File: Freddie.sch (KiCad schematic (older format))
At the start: 14 parts, among them J100 cond, J101 cond, U18 74LS08, U6 Freddie, Y1 Crystal

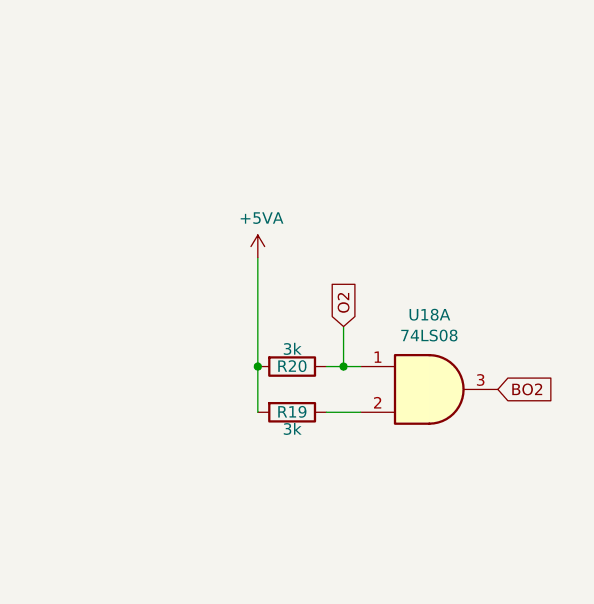
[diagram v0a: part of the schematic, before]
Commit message: GTIA
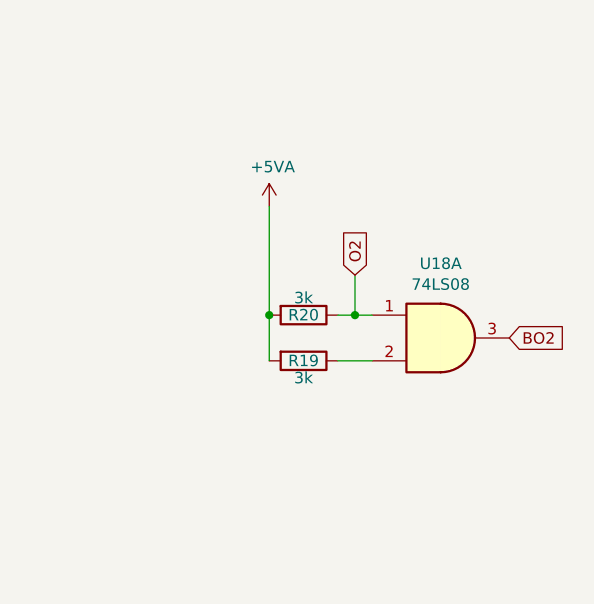
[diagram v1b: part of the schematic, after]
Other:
- moved on the sheet: R19, R20, U18A
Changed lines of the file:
@@
 $Descr A4 11693 8268
 encoding utf-8
-Sheet 5 13
+Sheet 5 14
 Title ""
 Date ""
@@
 L 74xx:74LS08 U18
 U 1 1 60220D8B
-P 8900 3025
-F 0 "U18" H 8900 3350 50  0000 C CNN
-F 1 "74LS08" H 8900 3259 50  0000 C CNN
-F 2 "Package_DIP:DIP-14_W7.62mm_Socket" H 8900 3025 50  0001 C CNN
-F 3 "http://www.ti.com/lit/gpn/sn74LS08" H 8900 3025 50  0001 C CNN
-	1    8900 3025
+P 8950 2800
+F 0 "U18" H 8950 3125 50  0000 C CNN
+F 1 "74LS08" H 8950 3034 50  0000 C CNN
+F 2 "Package_DIP:DIP-14_W7.62mm_Socket" H 8950 2800 50  0001 C CNN
+F 3 "http://www.ti.com/lit/gpn/sn74LS08" H 8950 2800 50  0001 C CNN
+	1    8950 2800
 	1    0    0    -1
 $EndComp
@@
 L Device:R R19
 U 1 1 602255FA
-P 8300 3125
-F 0 "R19" V 8300 3125 50  0000 C CNN
-F 1 "3k" V 8375 3125 50  0000 C CNN
-F 2 "Atari:R_Axial_DIN0207_L3.6mm_D2.2mm_P10.16mm_Horizontal" V 8230 3125 50  0001 C CNN
-F 3 "~" H 8300 3125 50  0001 C CNN
-	1    8300 3125
+P 8350 2900
+F 0 "R19" V 8350 2900 50  0000 C CNN
+F 1 "3k" V 8425 2900 50  0000 C CNN
+F 2 "Atari:R_Axial_DIN0207_L3.6mm_D2.2mm_P10.16mm_Horizontal" V 8280 2900 50  0001 C CNN
+F 3 "~" H 8350 2900 50  0001 C CNN
+	1    8350 2900
 	0    1    1    0
 $EndComp
@@
 L Device:R R20
 U 1 1 60225F1A
-P 8300 2925
-F 0 "R20" V 8300 2925 50  0000 C CNN
-F 1 "3k" V 8225 2925 50  0000 C CNN
-F 2 "Atari:R_Axial_DIN0207_L3.6mm_D2.2mm_P10.16mm_Horizontal" V 8230 2925 50  0001 C CNN
-F 3 "~" H 8300 2925 50  0001 C CNN
-	1    8300 2925
-	0    1    1    0
-$EndComp
-Wire Wire Line
-	8450 2925 8525 2925
-Text GLabel 9200 3025 2    50   Input ~ 0
+P 8350 2700
+F 0 "R20" V 8350 2700 50  0000 C CNN
+F 1 "3k" V 8275 2700 50  0000 C CNN
+F 2 "Atari:R_Axial_DIN0207_L3.6mm_D2.2mm_P10.16mm_Horizontal" V 8280 2700 50  0001 C CNN
+F 3 "~" H 8350 2700 50  0001 C CNN
+	1    8350 2700
+	0    1    1    0
+$EndComp
+Wire Wire Line
+	8500 2700 8575 2700
+Text GLabel 9250 2800 2    50   Input ~ 0
 BO2
 Wire Wire Line
-	8150 3125 8150 2925
+	8200 2900 8200 2700
 $Comp
 L power:+5VA #PWR0142
 U 1 1 602274F9
-P 8150 2450
-F 0 "#PWR0142" H 8150 2300 50  0001 C CNN
-F 1 "+5VA" H 8165 2623 50  0000 C CNN
-F 2 "" H 8150 2450 50  0001 C CNN
-F 3 "" H 8150 2450 50  0001 C CNN
-	1    8150 2450
-	1    0    0    -1
-$EndComp
-Wire Wire Line
-	8150 2450 8150 2925
-Connection ~ 8150 2925
-Text GLabel 8525 2750 1    50   Input ~ 0
+P 8200 2225
+F 0 "#PWR0142" H 8200 2075 50  0001 C CNN
+F 1 "+5VA" H 8215 2398 50  0000 C CNN
+F 2 "" H 8200 2225 50  0001 C CNN
+F 3 "" H 8200 2225 50  0001 C CNN
+	1    8200 2225
+	1    0    0    -1
+$EndComp
+Wire Wire Line
+	8200 2225 8200 2700
+Connection ~ 8200 2700
+Text GLabel 8575 2525 1    50   Input ~ 0
 O2
 Wire Wire Line
-	8450 3125 8600 3125
-Wire Wire Line
-	8525 2750 8525 2925
-Connection ~ 8525 2925
-Wire Wire Line
-	8525 2925 8600 2925
+	8500 2900 8650 2900
+Wire Wire Line
+	8575 2525 8575 2700
+Connection ~ 8575 2700
+Wire Wire Line
+	8575 2700 8650 2700
 $Comp
 L Connector_Generic:Conn_01x01 J100

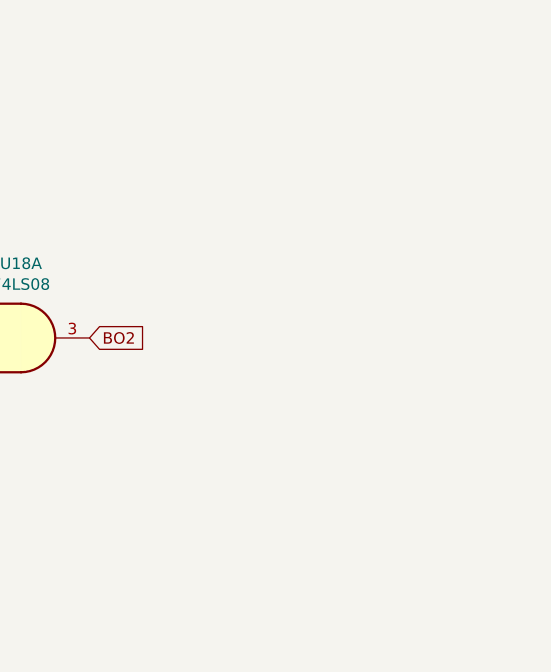
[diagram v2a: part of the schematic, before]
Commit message: Schema finished
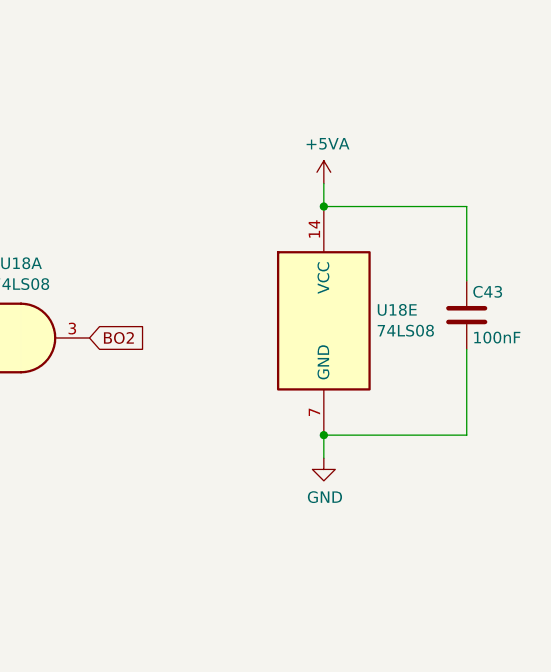
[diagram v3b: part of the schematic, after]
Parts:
- added C43: 100nF, Atari:C_Axial_L5.1mm_D2.5mm_P12.50mm_Horizontal, symbol Device:C
- added unit 5 of U18
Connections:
- net +5VA: now also C43.1, U18.14 (VCC)
- net GND: now also C43.2, U18.7 (GND)
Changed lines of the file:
@@
 	4200 1825 4200 2575
 Connection ~ 2950 1825
+$Comp
+L 74xx:74LS08 U18
+U 5 1 603127C5
+P 10275 2725
+F 0 "U18" H 10505 2771 50  0000 L CNN
+F 1 "74LS08" H 10505 2680 50  0000 L CNN
+F 2 "Package_DIP:DIP-14_W7.62mm_Socket" H 10275 2725 50  0001 C CNN
+F 3 "http://www.ti.com/lit/gpn/sn74LS08" H 10275 2725 50  0001 C CNN
+	5    10275 2725
+	1    0    0    -1
+$EndComp
+$Comp
+L power:+5VA #PWR0235
+U 1 1 60314A8A
+P 10275 2125
+F 0 "#PWR0235" H 10275 1975 50  0001 C CNN
+F 1 "+5VA" H 10290 2298 50  0000 C CNN
+F 2 "" H 10275 2125 50  0001 C CNN
+F 3 "" H 10275 2125 50  0001 C CNN
+	1    10275 2125
+	1    0    0    -1
+$EndComp
+Wire Wire Line
+	10275 2125 10275 2225
+$Comp
+L power:GND #PWR0236
+U 1 1 6031559C
+P 10275 3325
+F 0 "#PWR0236" H 10275 3075 50  0001 C CNN
+F 1 "GND" H 10280 3152 50  0000 C CNN
+F 2 "" H 10275 3325 50  0001 C CNN
+F 3 "" H 10275 3325 50  0001 C CNN
+	1    10275 3325
+	1    0    0    -1
+$EndComp
+Wire Wire Line
+	10275 3225 10275 3325
+$Comp
+L Device:C C43
+U 1 1 603176DF
+P 10900 2700
+F 0 "C43" H 10925 2800 50  0000 L CNN
+F 1 "100nF" H 10925 2600 50  0000 L CNN
+F 2 "Atari:C_Axial_L5.1mm_D2.5mm_P12.50mm_Horizontal" H 10938 2550 50  0001 C CNN
+F 3 "~" H 10900 2700 50  0001 C CNN
+	1    10900 2700
+	1    0    0    -1
+$EndComp
+Wire Wire Line
+	10275 2225 10900 2225
+Wire Wire Line
+	10900 2225 10900 2550
+Connection ~ 10275 2225
+Wire Wire Line
+	10275 3225 10900 3225
+Wire Wire Line
+	10900 3225 10900 2850
+Connection ~ 10275 3225
 $EndSCHEMATC

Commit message: Tracking
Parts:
- R18, R26: footprint Atari:R_Axial_DIN0207_L3.6mm_D2.2mm_P10.16mm_Horizontal -> Resistor_THT:R_Axial_DIN0207_L6.3mm_D2.5mm_P10.16mm_Horizontal
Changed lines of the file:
@@
 F 0 "R18" V 3843 1825 50  0000 C CNN
 F 1 "240" V 3934 1825 50  0000 C CNN
-F 2 "Atari:R_Axial_DIN0207_L3.6mm_D2.2mm_P10.16mm_Horizontal" V 3980 1825 50  0001 C CNN
+F 2 "Resistor_THT:R_Axial_DIN0207_L6.3mm_D2.5mm_P10.16mm_Horizontal" V 3980 1825 50  0001 C CNN
 F 3 "~" H 4050 1825 50  0001 C CNN
 	1    4050 1825
@@
 F 0 "R26" V 3843 2575 50  0000 C CNN
 F 1 "1M" V 3934 2575 50  0000 C CNN
-F 2 "Atari:R_Axial_DIN0207_L3.6mm_D2.2mm_P10.16mm_Horizontal" V 3980 2575 50  0001 C CNN
+F 2 "Resistor_THT:R_Axial_DIN0207_L6.3mm_D2.5mm_P10.16mm_Horizontal" V 3980 2575 50  0001 C CNN
 F 3 "~" H 4050 2575 50  0001 C CNN
 	1    4050 2575

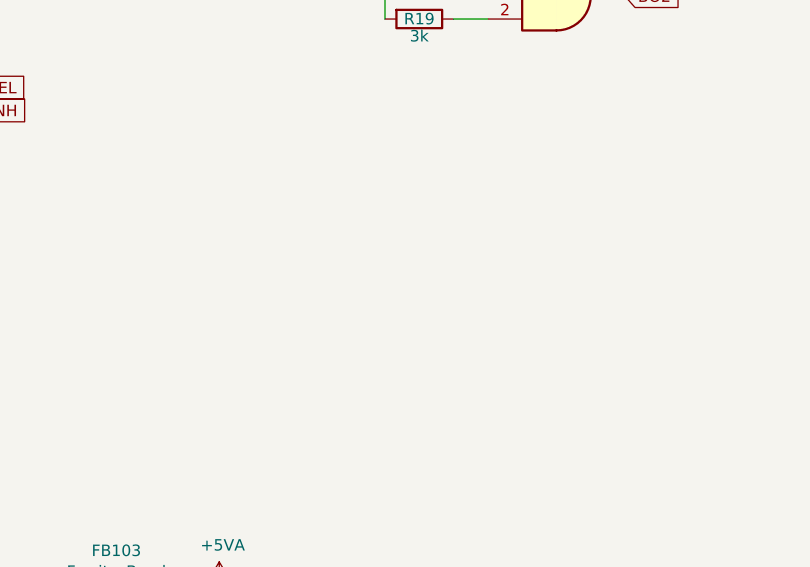
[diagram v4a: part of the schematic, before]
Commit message: Trackimg
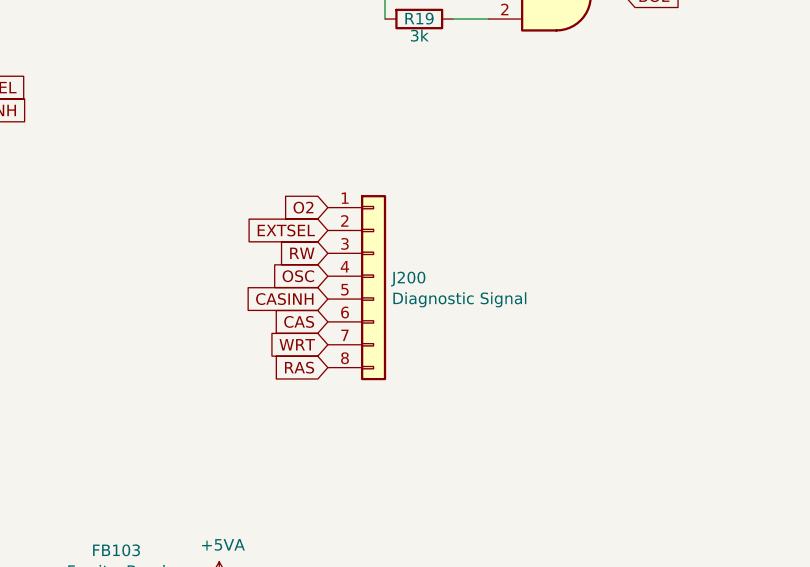
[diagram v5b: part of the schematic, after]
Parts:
- added J200: Diagnostic Signal, Connector_PinHeader_2.54mm:PinHeader_1x08_P2.54mm_Vertical, symbol Connector_Generic:Conn_01x08
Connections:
- net CAS: now also J200.6 (Pin_6)
- net CASINH: now also J200.5 (Pin_5)
- net EXTSEL: now also J200.2 (Pin_2)
- net O2: now also J200.1 (Pin_1)
- net OSC: now also J200.4 (Pin_4)
- net RAS: now also J200.8 (Pin_8)
- net RW: now also J200.3 (Pin_3)
- net WRT: now also J200.7 (Pin_7)
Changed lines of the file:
@@
 	10900 3225 10900 2850
 Connection ~ 10275 3225
+$Comp
+L Connector_Generic:Conn_01x08 J200
+U 1 1 60415DC7
+P 8150 4025
+F 0 "J200" H 8230 4017 50  0000 L CNN
+F 1 "Diagnostic Signal" H 8230 3926 50  0000 L CNN
+F 2 "Connector_PinHeader_2.54mm:PinHeader_1x08_P2.54mm_Vertical" H 8150 4025 50  0001 C CNN
+F 3 "~" H 8150 4025 50  0001 C CNN
+	1    8150 4025
+	1    0    0    -1
+$EndComp
+Text GLabel 7950 4225 0    50   Input ~ 0
+CAS
+Text GLabel 7950 4325 0    50   Input ~ 0
+WRT
+Text GLabel 7950 4425 0    50   Input ~ 0
+RAS
+Text GLabel 7950 3925 0    50   Input ~ 0
+RW
+Text GLabel 7950 4025 0    50   Input ~ 0
+OSC
+Text GLabel 7950 3725 0    50   Input ~ 0
+O2
+Text GLabel 7950 4125 0    50   Input ~ 0
+CASINH
+Text GLabel 7950 3825 0    50   Input ~ 0
+EXTSEL
 $EndSCHEMATC

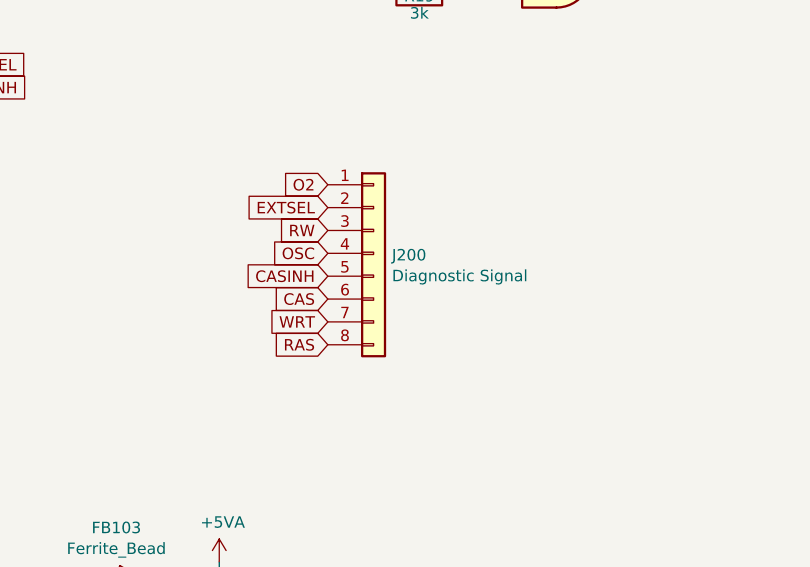
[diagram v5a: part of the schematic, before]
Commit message: Diagnostic
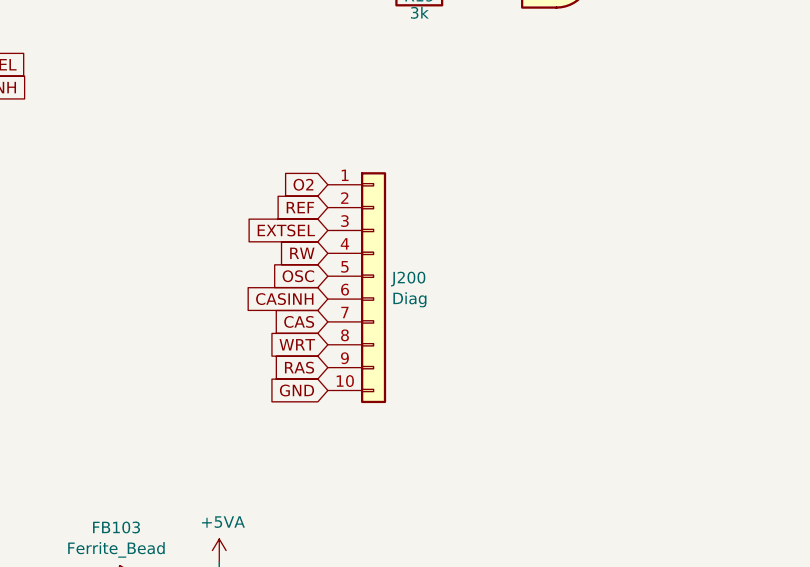
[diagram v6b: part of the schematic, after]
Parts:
- removed J200: Diagnostic Signal, Connector_PinHeader_2.54mm:PinHeader_1x08_P2.54mm_Vertical, symbol Connector_Generic:Conn_01x08
- added J200: Diag, Connector_PinHeader_2.54mm:PinHeader_1x10_P2.54mm_Vertical, symbol Connector_Generic:Conn_01x10
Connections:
- net CAS: now also J200.7 (Pin_7)
- net CASINH: now also J200.6 (Pin_6)
- net EXTSEL: now also J200.3 (Pin_3)
- net GND: now also J200.10 (Pin_10)
- net O2: now also J200.1 (Pin_1)
- net OSC: now also J200.5 (Pin_5)
- net RAS: now also J200.9 (Pin_9)
- net RW: now also J200.4 (Pin_4)
- net WRT: now also J200.8 (Pin_8)
- new net REF: J200.2 (Pin_2)
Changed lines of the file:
@@
 	10900 3225 10900 2850
 Connection ~ 10275 3225
-$Comp
-L Connector_Generic:Conn_01x08 J200
-U 1 1 60415DC7
-P 8150 4025
-F 0 "J200" H 8230 4017 50  0000 L CNN
-F 1 "Diagnostic Signal" H 8230 3926 50  0000 L CNN
-F 2 "Connector_PinHeader_2.54mm:PinHeader_1x08_P2.54mm_Vertical" H 8150 4025 50  0001 C CNN
-F 3 "~" H 8150 4025 50  0001 C CNN
-	1    8150 4025
-	1    0    0    -1
-$EndComp
-Text GLabel 7950 4225 0    50   Input ~ 0
+Text GLabel 7950 4325 0    50   Input ~ 0
 CAS
-Text GLabel 7950 4325 0    50   Input ~ 0
+Text GLabel 7950 4425 0    50   Input ~ 0
 WRT
-Text GLabel 7950 4425 0    50   Input ~ 0
+Text GLabel 7950 4525 0    50   Input ~ 0
 RAS
-Text GLabel 7950 3925 0    50   Input ~ 0
+Text GLabel 7950 4025 0    50   Input ~ 0
 RW
-Text GLabel 7950 4025 0    50   Input ~ 0
+Text GLabel 7950 4125 0    50   Input ~ 0
 OSC
 Text GLabel 7950 3725 0    50   Input ~ 0
 O2
-Text GLabel 7950 4125 0    50   Input ~ 0
+Text GLabel 7950 4225 0    50   Input ~ 0
 CASINH
+Text GLabel 7950 3925 0    50   Input ~ 0
+EXTSEL
+$Comp
+L Connector_Generic:Conn_01x10 J200
+U 1 1 60423A62
+P 8150 4125
+F 0 "J200" H 8230 4117 50  0000 L CNN
+F 1 "Diag" H 8230 4026 50  0000 L CNN
+F 2 "Connector_PinHeader_2.54mm:PinHeader_1x10_P2.54mm_Vertical" H 8150 4125 50  0001 C CNN
+F 3 "~" H 8150 4125 50  0001 C CNN
+	1    8150 4125
+	1    0    0    -1
+$EndComp
 Text GLabel 7950 3825 0    50   Input ~ 0
-EXTSEL
+REF
+Text GLabel 7950 4625 0    50   Input ~ 0
+GND
 $EndSCHEMATC
